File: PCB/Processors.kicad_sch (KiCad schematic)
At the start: 0 parts

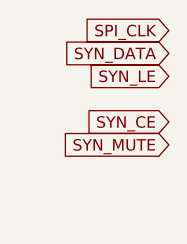
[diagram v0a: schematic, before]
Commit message: new file:   Datasheet/HMC849A_RF_Switch_SPDT.pdf 	new file:   Datasheet/TG2016SMN_26MHz_MCGNNM_Oscillator.pdf 	modified:   PCB/DroidRadio.kicad_pro 	modified:   PCB/DroidRadio.kicad_sch 	modified:   PCB/Processors.kicad_sch 	modified:   PCB/Simulation/Transmitter_Side.pll 	modified:   PCB/Transmitter.kicad_sch 	deleted:    PCB/~DroidRadio.kicad_pro.lck
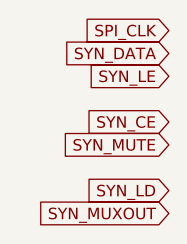
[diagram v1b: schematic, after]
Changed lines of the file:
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@@
 	(generator_version "10.0")
 	(paper "A4")
+	(global_label "SYN_LD"
+		(shape input)
+		(at 66.04 67.31 180)
+		(fields_autoplaced yes)
+		(effects
+			(font
+				(size 1.27 1.27)
+			)
+			(justify right)
+		)
+		(property "Intersheetrefs" "${INTERSHEET_REFS}"
+			(at 56.1605 67.31 0)
+			(hide yes)
+			(show_name no)
+			(do_not_autoplace no)
+			(effects
+				(font
+					(size 1.27 1.27)
+				)
+				(justify right)
+			)
+		)
+	)
 	(global_label "SYN_CE"
 		(shape input)
@@
 			(hide yes)
 			(show_name no)
+			(do_not_autoplace no)
+			(effects
+				(font
+					(size 1.27 1.27)
+				)
+				(justify right)
+			)
+		)
+	)
+	(global_label "SYN_MUXOUT"
+		(shape input)
+		(at 66.04 69.85 180)
+		(fields_autoplaced yes)
+		(effects
+			(font
+				(size 1.27 1.27)
+			)
+			(justify right)
+		)
+		(property "Intersheetrefs" "${INTERSHEET_REFS}"
+			(at 50.8386 69.85 0)
+			(hide yes)
+			(show_name no)
